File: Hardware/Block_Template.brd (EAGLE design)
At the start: 41.7 x 35.6 mm, 4 parts, among them J1 EDISON_CONNECTOR_FULLMOUNTING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, J2 EDISON_CONNECTOR_FULLHEADER

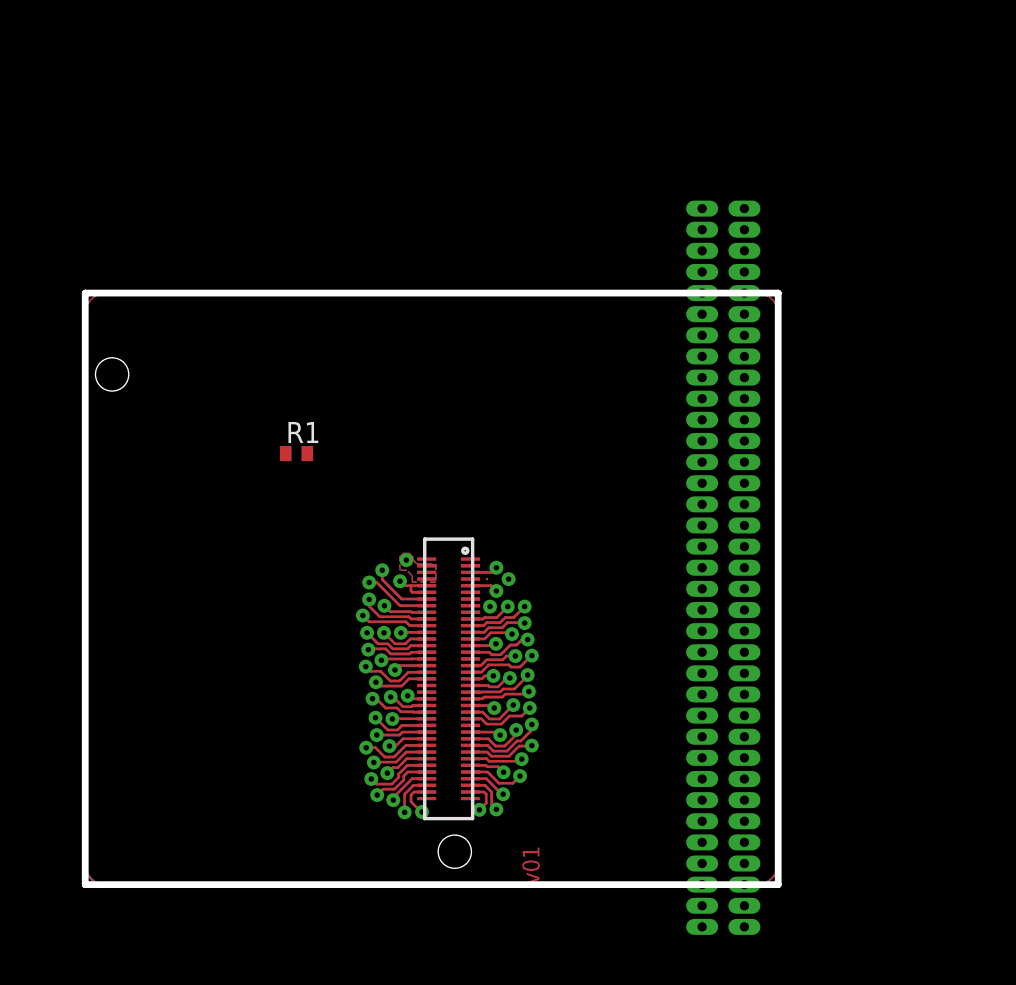
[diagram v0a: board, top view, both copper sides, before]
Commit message: ready for manufacture
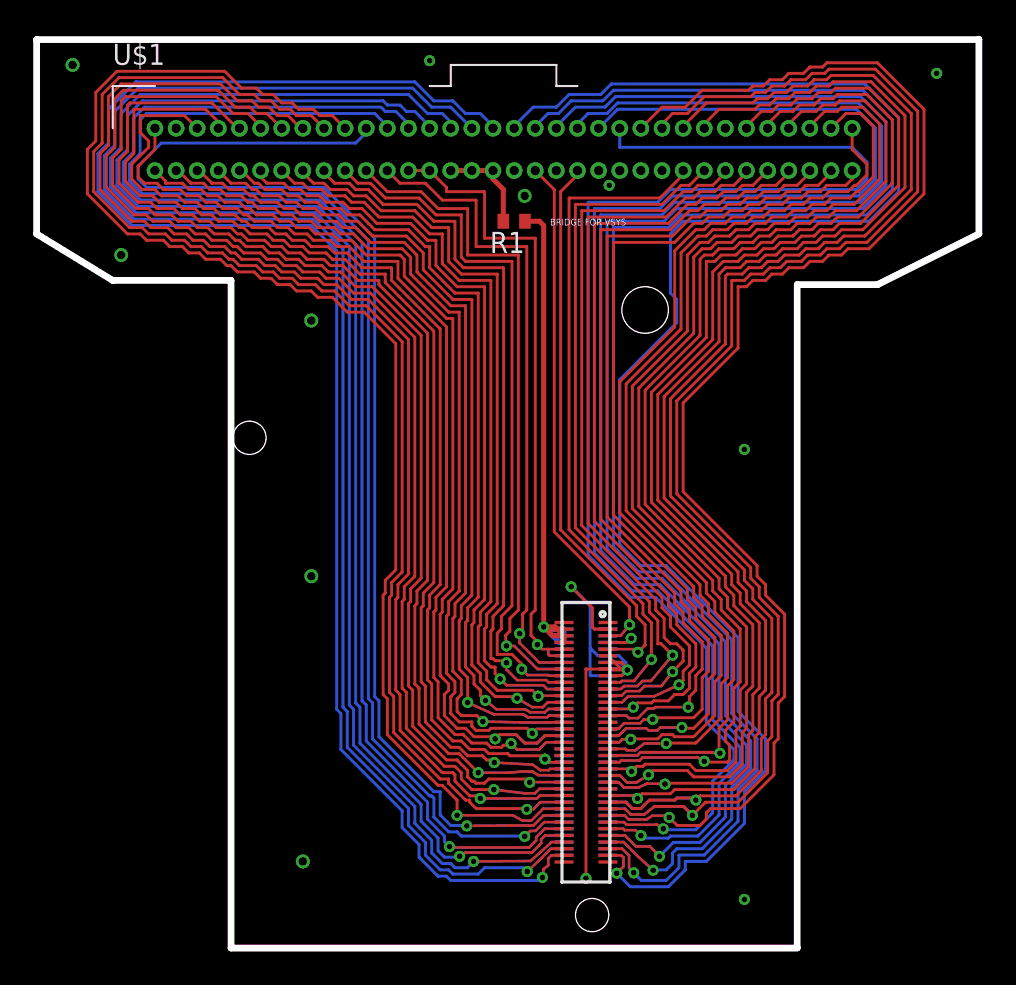
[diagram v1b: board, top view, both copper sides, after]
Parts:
- moved U$1 28.1 mm to (28.6, 48.0), flipped to the top, turned to 0 degrees
- moved R1 19.1 mm to (28.6, 43.7), turned to 180 degrees
- moved J2 9.09 mm to (32.9, 12.4)
- moved J1 9.09 mm to (36.2, 0.00)
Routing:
- net FW_RCVR: track 4.20 -> 100.5 mm
- net OSC_CLK_OUT: track 5.19 -> 99.3 mm
- net GP81_SD_0_DAT1: track 4.68 -> 97.2 mm
- net GP128_UART_1_CTS: track 4.68 -> 96.8 mm
- net GP80_SD_0_DAT0: track 5.27 -> 95.2 mm
- net GP83_SD_0_DAT3: track 5.27 -> 94.7 mm
- net GP129_UART_1_RTS: track 6.86 -> 94.1 mm
- net GP82_SD_0_DAT2: track 7.36 -> 93.3 mm
- net GP130_UART_1_RX: track 4.30 -> 89.4 mm
- net GP79_SD_0_CMD: track 8.08 -> 90.9 mm
- net GP43_I2S_2_TXD: track 8.31 -> 89.8 mm
- net GP114_SPI_2_RXD: track 6.38 -> 86.8 mm
- net GP115_SPI_2_TXD: track 8.10 -> 87.6 mm
- net GP77_SD_0_CD#: track 5.45 -> 83.0 mm
- net GP109_SPI_2_CLK: track 9.36 -> 86.8 mm
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- removed copper zone on layer 1, net VSYS
- removed copper zone on layer 16, net VSYS
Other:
- board size 41.7 x 35.6 mm -> 56.6 x 54.6 mm
- board text added: "BRIDGE FOR VSYS"
- board text removed: "4xM2.0"
- board text removed: "v01"
